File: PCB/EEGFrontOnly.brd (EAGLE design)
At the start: 83 x 44.9 mm, 102 parts, among them IC1 ADS1299-X, IC2 ADUM3151-3, U1 LP2985-33DBVT, U10 ISO721D, U2 B0505S-1WB0505S-1W, U3 TPS60403DBVT, U4 TPS73225DBVR, U5 TPS73225DBVR, U6 TPD4E1B06DCKR, U7 TPD4E1B06DCKR, U8 TPD4E1B06DCKR, U9 HT7333

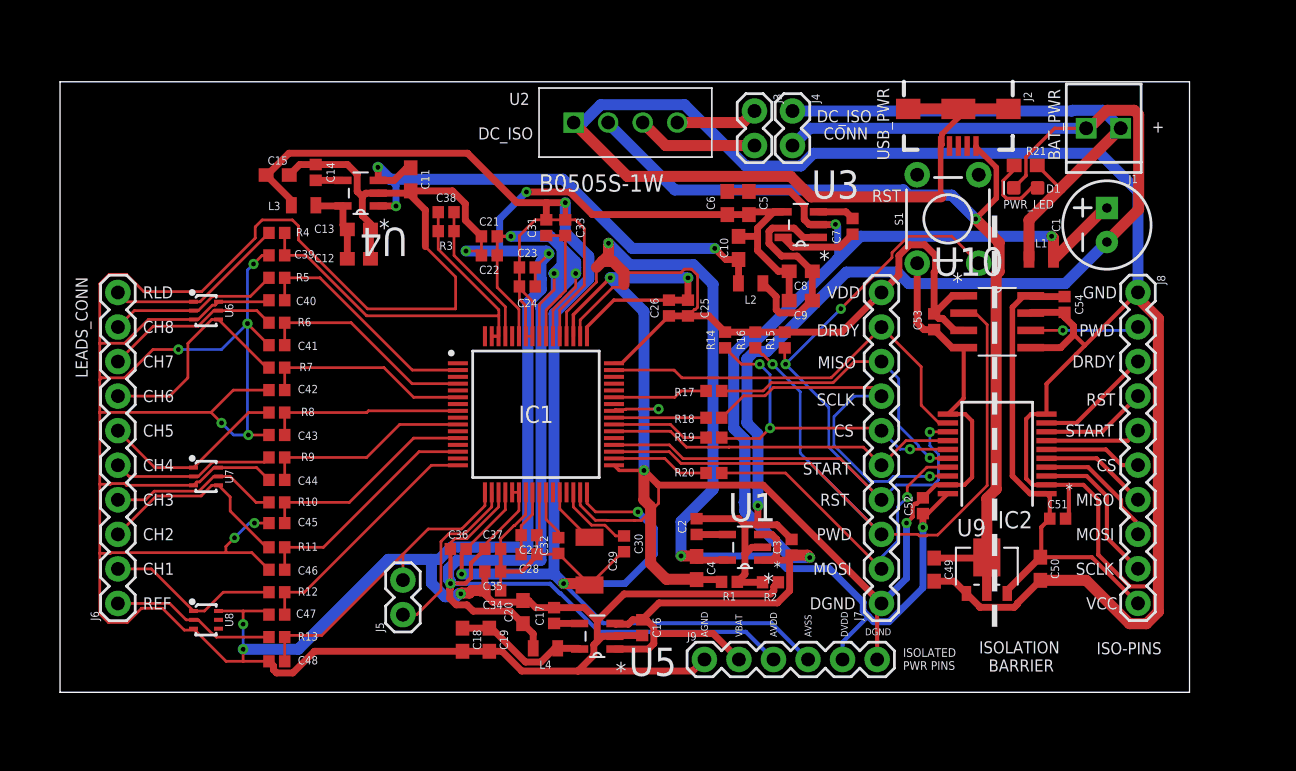
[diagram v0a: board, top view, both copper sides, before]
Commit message: front only PCB complete!
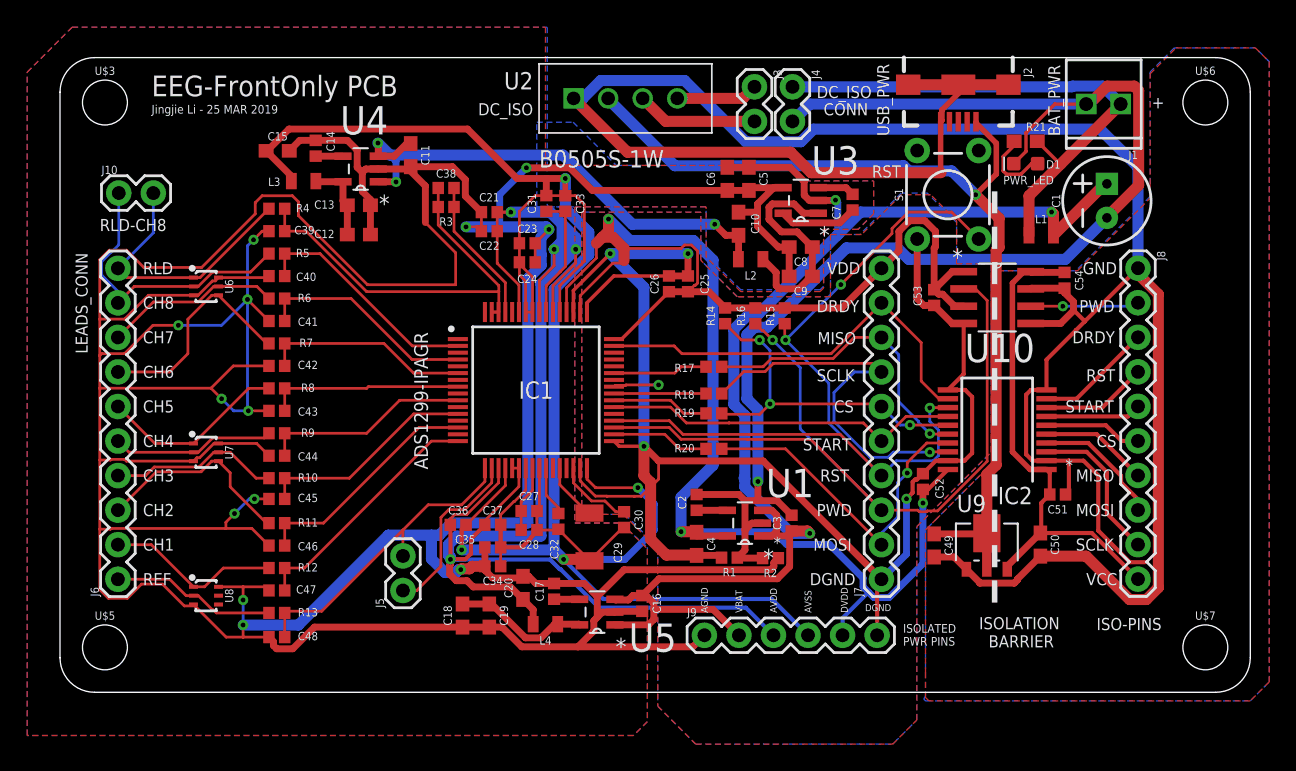
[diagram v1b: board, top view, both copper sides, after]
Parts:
- added J10: (no value), SparkFun-Connectors:1X02
- added U$3, U$5, U$6, U$7: (no value), SparkFun-Hardware:STAND-OFF
- moved C1 1.78 mm to (77.0, 36.1)
- moved U2 1.78 mm to (37.8, 43.7)
- moved C12 1.78 mm to (22.0, 33.6)
- moved C25 1.78 mm to (46.2, 30.0)
- moved C26 1.78 mm to (44.8, 30.0)
- moved C40 1.78 mm to (15.9, 30.6)
- moved C41 1.78 mm to (15.9, 27.3)
- moved C53 1.78 mm to (64.3, 29.0)
- moved C9 1.78 mm to (54.5, 30.6)
- moved L1 1.78 mm to (72.1, 33.6)
- moved L2 1.78 mm to (50.8, 31.8)
- moved R17 1.78 mm to (48.1, 23.9)
- moved R6 1.78 mm to (15.9, 28.9)
- moved U10 1.78 mm to (68.9, 29.0)
- moved U6 1.78 mm to (10.7, 29.8)
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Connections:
- net P_BIAS: now also J10.2
- net P_IN8: now also J10.1
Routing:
- net P_IN8: track 12.6 -> 21.7 mm
- net P_BIAS: track 13.5 -> 20.1 mm
- added copper zone on layer 1, net AGND
- added copper zone on layer 16, net AGND
- added copper zone on layer 1, net DGND
- added copper zone on layer 16, net DGND
- added copper zone on layer 1, net GND-ISO
- added copper zone on layer 16, net GND-ISO
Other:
- board size 83 x 44.9 mm -> 87.5 x 46.7 mm
- board text added: "ADS1299-IPAGR"
- board text added: "EEG-FrontOnly PCB"
- board text added: "Jingjie Li - 25 MAR 2019"
- board text added: "RLD-CH8"
